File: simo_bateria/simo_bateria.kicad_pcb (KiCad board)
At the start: 2 copper layers, 23 x 88 mm, 4 parts, among them J1 conector salida, U1 simo_bateria, U2 cargador_bateria, U3 conversor_dc

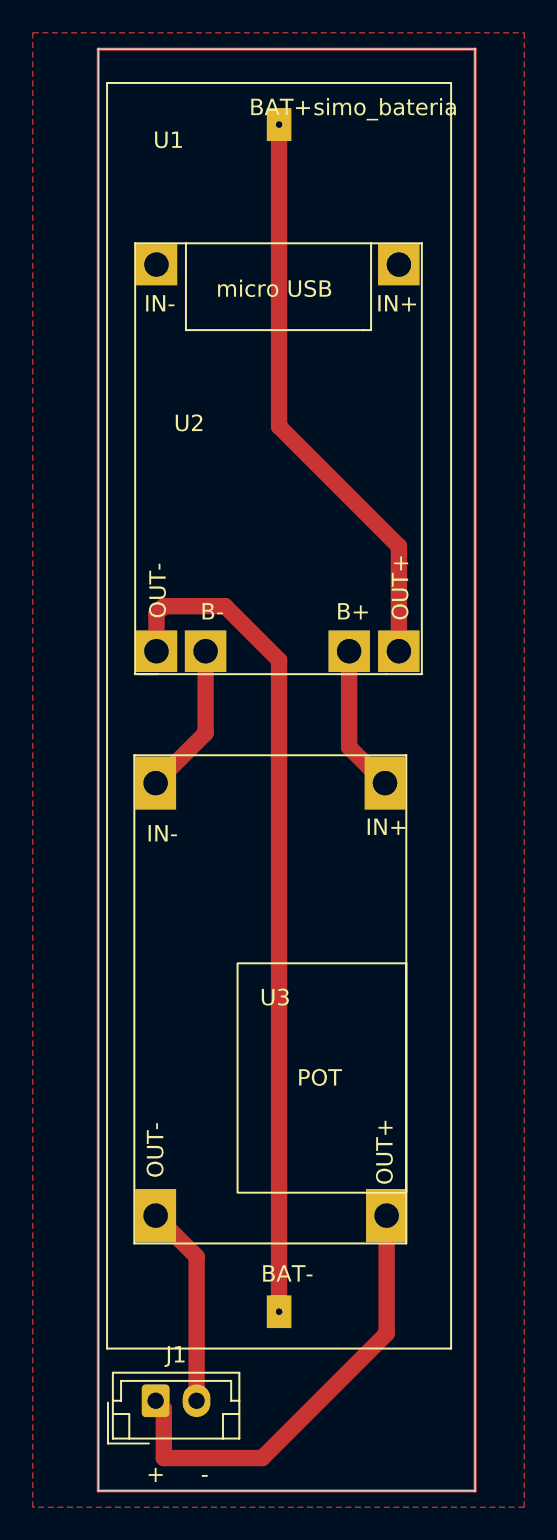
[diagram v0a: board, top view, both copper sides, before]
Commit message: se actualizo la placa bateria
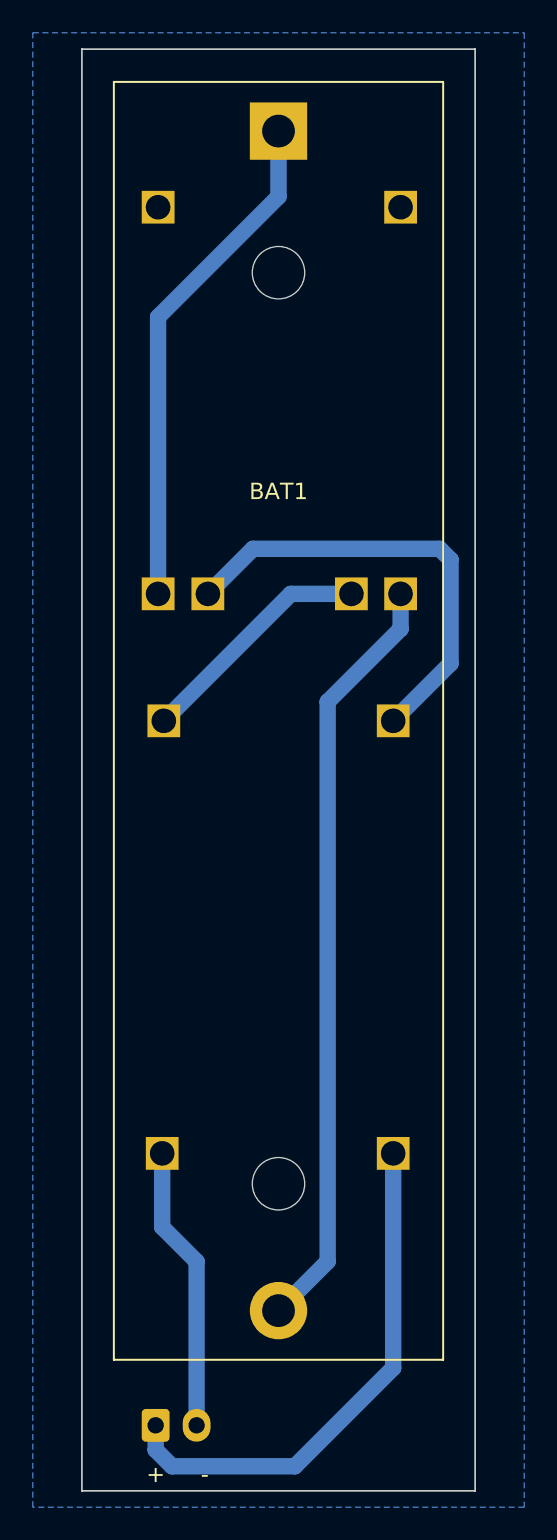
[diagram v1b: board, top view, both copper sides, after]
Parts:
- removed U1: simo_bateria, simo_bateria:bateria
- added BAT1: bateria, Battery:BatteryHolder_MPD_BH-18650-PC2, F.Cu at (130.0, 31.0)
- J1, U2, U3: moved to B.Cu
- moved U2 15.3 mm to (137.4, 35.6), turned to 180 degrees
- moved U3 15.0 mm to (137.0, 67.0), turned to 180 degrees
- moved J1 1.50 mm to (122.5, 110.0)
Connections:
- J1 pad 1: +3V3 -> +BATT
- U3 pad 1: Net-(U2-Pad3) -> Net-(U2-Pad5)
- U3 pad 2: GND -> +BATT
- U3 pad 3: Net-(U2-Pad5) -> Net-(U2-Pad3)
- U3 pad 4: +3V3 -> GND
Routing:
- net +BATT: track 0.00 -> 32.0 mm
- net +3V3: track 27.7 -> 0.00 mm
- net Net-(U2-Pad5): track 8.96 -> 27.5 mm
- net Net-(U2-Pad3): track 9.31 -> 14.7 mm
- net GND: track 12.3 -> 17.5 mm
- net Net-(BAT1-Pad2): track 51.1 -> 46.8 mm
- net Net-(BAT1-Pad1): track 35.2 -> 31.3 mm
- added copper zone on B.Cu, net GND
- removed copper zone on F.Cu, net GND
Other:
- board size 23 x 88 mm -> 24 x 88 mm
